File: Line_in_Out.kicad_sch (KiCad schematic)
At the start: 10 parts, among them J4 Out Left, J5 Out Right

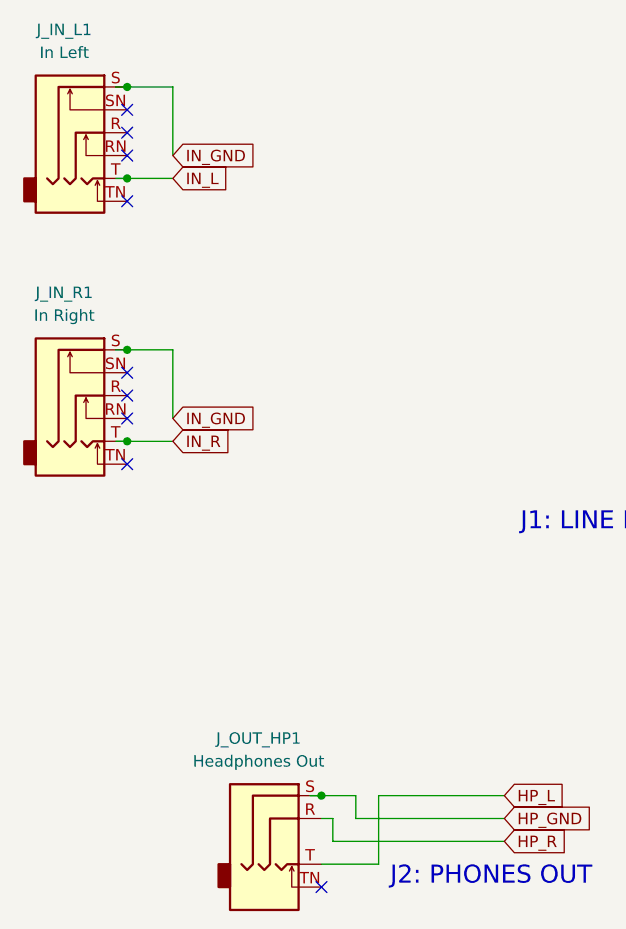
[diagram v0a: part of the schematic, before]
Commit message: Solve all warnings
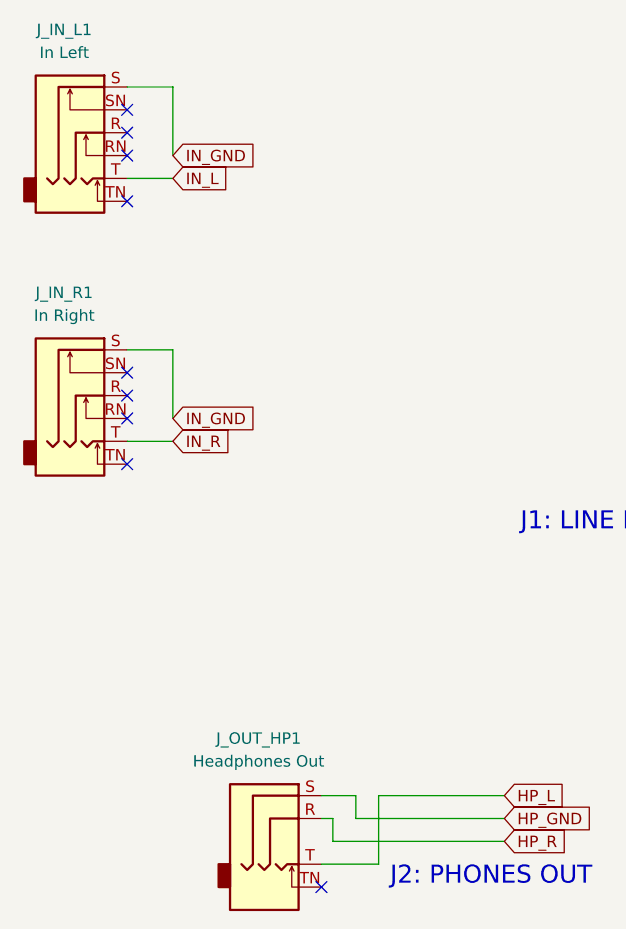
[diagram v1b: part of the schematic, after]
